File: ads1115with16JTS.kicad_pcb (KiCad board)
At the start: 2 copper layers, 127 x 152.4 mm, 41 parts, among them J1 Conn_01x02_Pin, J10 Conn_01x02_Pin, J11 Conn_01x02_Pin, J12 Conn_01x02_Pin, J13 Conn_01x02_Pin, J14 Conn_01x02_Pin, J15 Conn_01x02_Pin, J16 Conn_01x02_Pin, J17 Conn_01x04_Pin, J2 Conn_01x02_Pin, J3 Conn_01x02_Pin, J4 Conn_01x02_Pin, J5 Conn_01x02_Pin, J6 Conn_01x02_Pin, J7 Conn_01x02_Pin, J8 Conn_01x02_Pin, J9 Conn_01x02_Pin, U1 ADS1115IDGS, U2 ADS1115IDGS, U3 ADS1115IDGS, U4 ADS1115IDGS

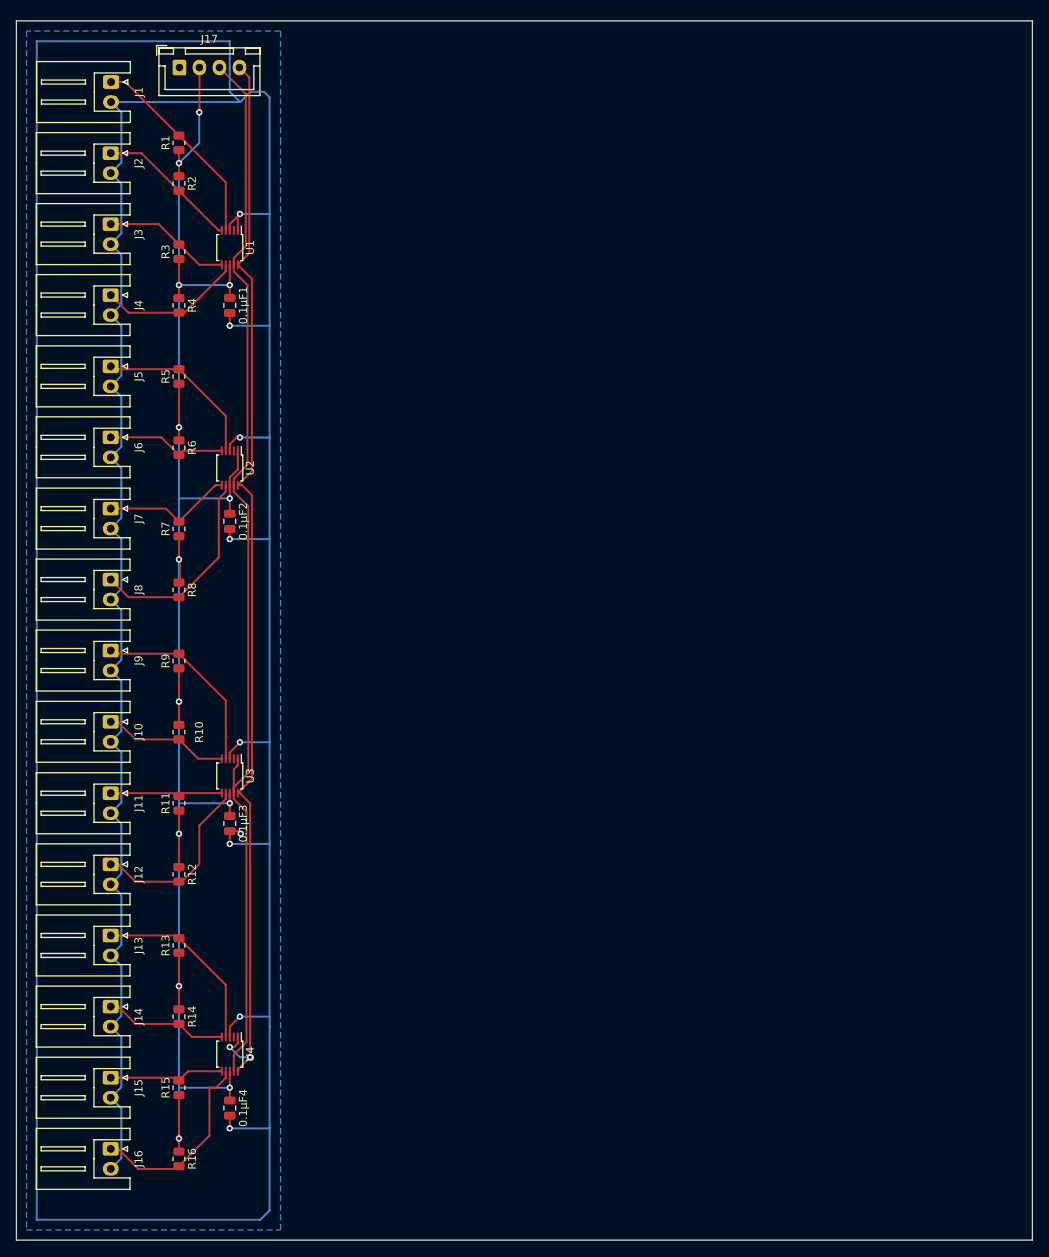
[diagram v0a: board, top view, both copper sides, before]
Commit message: snapshot v0.0.10
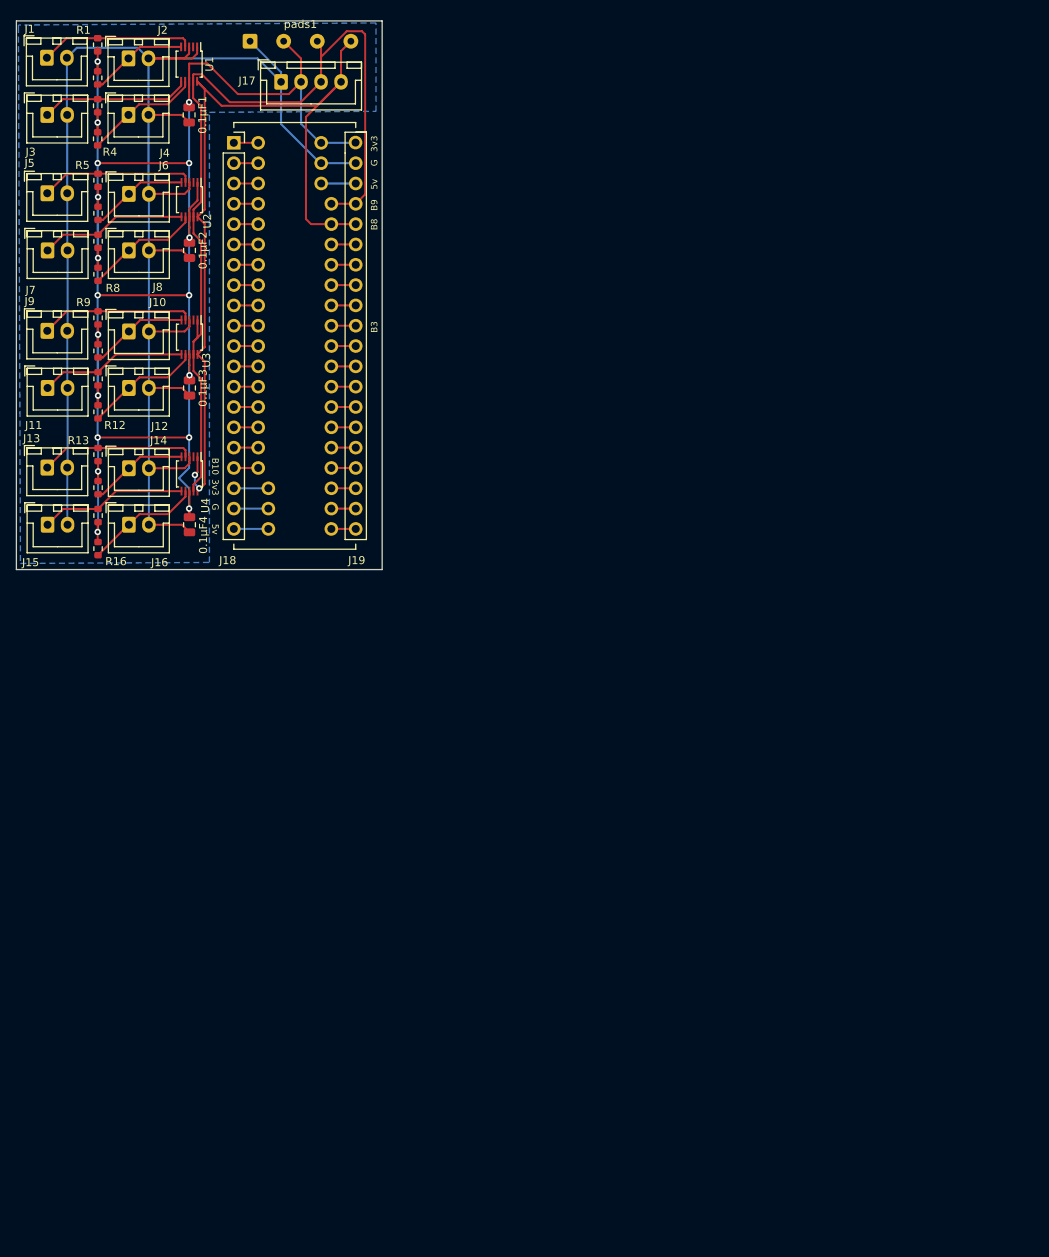
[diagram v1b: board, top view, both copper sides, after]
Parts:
- added J18: PinSocket_1x20_P2.54mm_Vertical, PG:b_pill_socket_1-20, F.Cu at (78.0, 64.8)
- added J18b1: SolderWire-0.25sqmm_1x20_P4.2mm_D0.65mm_OD1.7mm, PG:b_pill_takeoffPads_1-20, F.Cu at (86.1, 64.8)
- added J19: PinSocket_1x20_P2.54mm_Vertical, PG:b_pill_socket_21-40, F.Cu at (93.2, 64.8)
- added J19b1: SolderWire-0.25sqmm_1x20_P4.2mm_D0.65mm_OD1.7mm, PG:b_pill_takeoffPads_21-40, F.Cu at (90.2, 64.8)
- added pads1: SolderWire-0.25sqmm_1x04_P4.2mm_D0.65mm_OD1.7mm, Connector_Wire:SolderWire-0.25sqmm_1x04_P4.2mm_D0.65mm_OD1.7mm, F.Cu at (80.0, 27.9)
- J1, J10, J11, J12, J13, J14, J15, J16, J2, J3, J4, J5, J6, J7, J8, J9: footprint Connector_JST:JST_XH_S2B-XH-A_1x02_P2.50mm_Horizontal -> Connector_JST:JST_XH_B2B-XH-A_1x02_P2.50mm_Vertical
- R1, R10, R11, R12, R13, R14, R15, R16, R2, R3, R4, R5, R6, R7, R8, R9: footprint Resistor_SMD:R_0805_2012Metric -> Resistor_SMD:R_0603_1608Metric
- moved J16 78.0 mm to (64.9, 88.4), turned to 0 degrees
- moved R16 76.9 mm to (61.0, 91.4)
- moved 0.1µF4 73.1 mm to (72.4, 88.4)
- moved U4 72.7 mm to (72.4, 82.0)
- moved R15 72.2 mm to (61.0, 87.2)
- moved J15 69.6 mm to (54.7, 88.4), turned to 0 degrees
- moved J14 67.3 mm to (64.9, 81.3), turned to 0 degrees
- moved R14 66.9 mm to (61.0, 83.7)
- moved R13 62.2 mm to (61.0, 79.6)
- moved J12 59.6 mm to (64.9, 71.3), turned to 0 degrees
- moved J13 59.0 mm to (54.7, 81.2), turned to 0 degrees
- moved R12 58.7 mm to (61.0, 74.3)
- moved U3 55.1 mm to (72.4, 64.9)
- moved 0.1µF3 54.7 mm to (72.4, 71.3)
- moved R11 54.0 mm to (61.0, 70.1)
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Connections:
- net Net-(J17-Pin_3) renamed /SDA1
- net Net-(J17-Pin_4) renamed /SCL1
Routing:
- net GND: track 574.0 -> 222.8 mm, vias 9 -> 0
- net /SCL1: track 136.3 -> 109.3 mm
- net /SDA1: track 136.2 -> 115.3 mm
- net Net-(J8-Pin_1): track 25.9 -> 14.7 mm
- net Net-(J16-Pin_1): track 24.5 -> 14.7 mm
- net Net-(J12-Pin_1): track 23.1 -> 14.7 mm
- net +3V3: track 232.1 -> 240.5 mm, vias 13 -> 18
- net Net-(J1-Pin_1): track 25.5 -> 19.2 mm
- net Net-(J2-Pin_1): track 17.9 -> 12.4 mm
- net Net-(J9-Pin_1): track 24.2 -> 19.2 mm
- net Net-(J18-G): track 0.00 -> 4.45 mm
- net Net-(J18-5v): track 0.00 -> 4.45 mm
- net Net-(J18-3v3): track 0.00 -> 4.45 mm
- net Net-(J11-Pin_1): track 14.2 -> 18.5 mm
- net Net-(J13-Pin_1): track 23.4 -> 19.2 mm
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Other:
- board size 127 x 152.4 mm -> 45.7 x 68.6 mm
